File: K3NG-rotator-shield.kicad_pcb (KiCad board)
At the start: 2 copper layers, 81.9 x 70.1 mm, 25 parts, among them J1 Conn_01x08_Socket, J10 Conn_01x01_Pin, J11 Conn_01x10_Socket, J12 Conn_01x01_Pin, J13 Conn_01x01_Pin, J14 Conn_01x01_Pin, J15 Conn_01x01_Pin, J2 Conn_01x04_Socket, J3 Conn_01x02_Pin, J4 Conn_01x04_Socket, J5 Conn_01x01_Pin, J6 Conn_01x07_Socket, J7 Conn_01x06_Socket, J8 Conn_01x08_Socket, J9 Conn_01x06_Socket, U1 DRV8251ADDAR, U2 DRV8251ADDAR

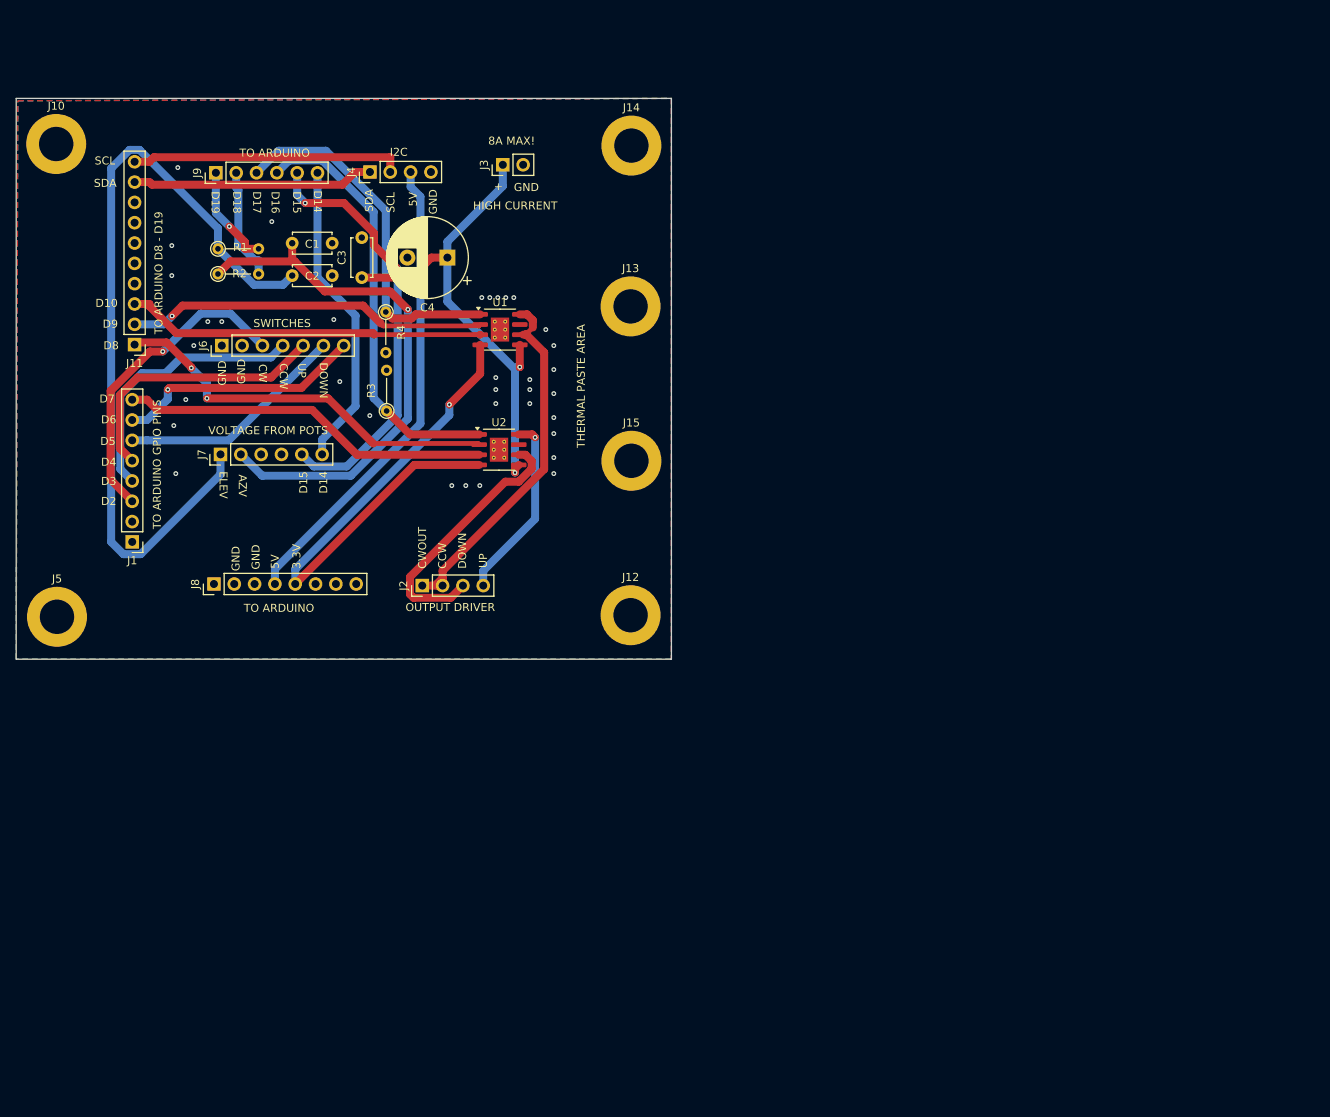
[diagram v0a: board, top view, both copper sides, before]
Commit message: Add files via upload
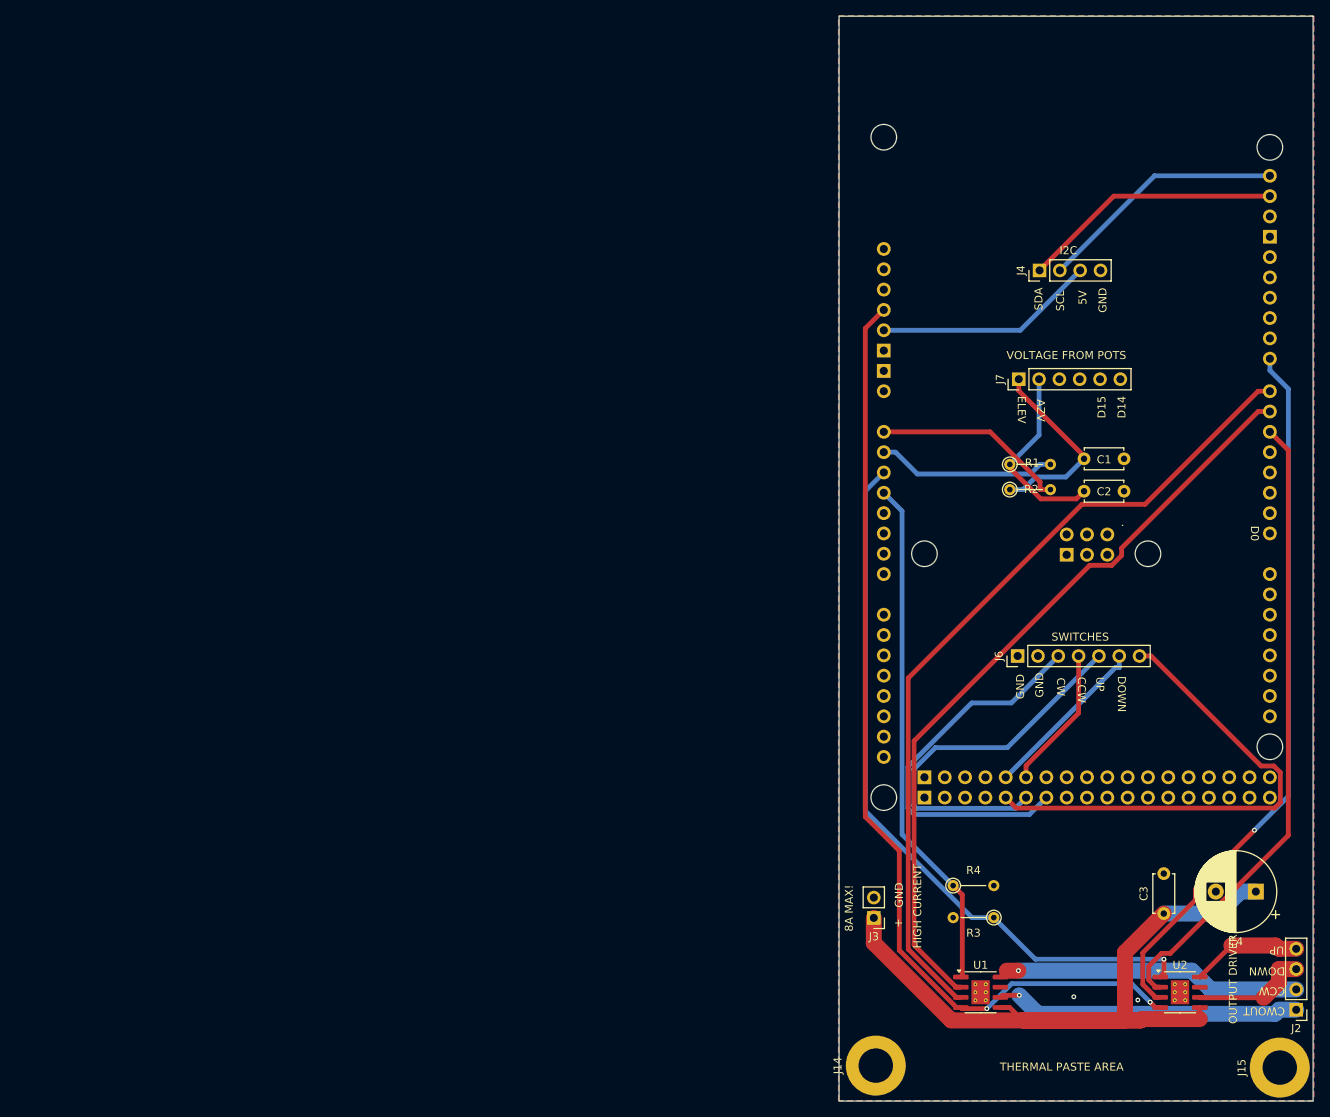
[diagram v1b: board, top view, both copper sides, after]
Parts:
- removed J1, J8: Conn_01x08_Socket, Connector_PinHeader_2.54mm:PinHeader_1x08_P2.54mm_Vertical
- removed J10, J12, J13, J5: Conn_01x01_Pin, MountingHole:MountingHole_4.3mm_M4_DIN965_Pad
- removed J11: Conn_01x10_Socket, Connector_PinHeader_2.54mm:PinHeader_1x10_P2.54mm_Vertical
- removed J9: Conn_01x06_Socket, Connector_PinHeader_2.54mm:PinHeader_1x06_P2.54mm_Vertical
- added A1: Arduino_Mega2560_R3_Shield, sparkfun-electromech:Arduino_Mega2560_R3_K3NG, F.Cu at (131.7, 25.0)
- moved C4 128.4 mm to (180.8, 133.2)
- moved C3 127.9 mm to (169.2, 136.0)
- moved J2 121.4 mm to (185.8, 148.0), turned to 180 degrees
- moved J14 119.0 mm to (133.2, 155.0), turned to 90 degrees
- moved J15 111.0 mm to (183.8, 155.2), turned to 90 degrees
- moved U2 108.8 mm to (171.3, 145.8)
- moved J6 106.8 mm to (151.0, 103.8)
- moved J3 104.9 mm to (133.0, 136.5), turned to 180 degrees
- moved C1 102.6 mm to (159.3, 79.2)
- moved C2 102.6 mm to (159.3, 83.2)
- moved R1 102.6 mm to (150.0, 79.8)
- moved R2 102.6 mm to (150.0, 83.0)
- moved U1 102.3 mm to (146.4, 145.8)
- moved R4 100.8 mm to (142.9, 132.5), turned to 0 degrees
- moved J7 100.2 mm to (151.1, 69.2)
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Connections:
- J2 pad 1: RotateCCW-OUT -> RotateCW-OUT
- J7 pad 1: /ElevationV -> /AzimuthV
- J7 pad 2: /AzimuthV -> /ElevationV
- J7 pad 5: Net-(J7-Pin_5) -> unconnected-(J7-Pin_5-Pad5)
- J7 pad 6: /ACD0 -> unconnected-(J7-Pin_6-Pad6)
- U1 pad 6: RotateCCW-OUT -> RotateCW-OUT
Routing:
- net /ElevationV: track 100.2 -> 23.9 mm
- net RotateCW: track 44.9 -> 103.0 mm
- net Net-(J7-Pin_5): track 53.6 -> 0.00 mm, vias 2 -> 0
- net Vref: track 68.6 -> 120.9 mm, vias 1 -> 2
- net RotateCCW: track 45.3 -> 95.6 mm, vias 1 -> 0
- net VM: track 61.2 -> 108.6 mm, vias 2 -> 0
- net /AzimuthV: track 67.8 -> 24.2 mm, vias 1 -> 0
- net RotateDown: track 46.2 -> 89.6 mm, vias 0 -> 1
- net /ACD0: track 38.9 -> 0.00 mm
- net RotateCW-OUT: track 0.00 -> 38.2 mm, vias 0 -> 1
- net IPRO1: track 53.8 -> 90.7 mm, vias 0 -> 1
- net 5V: track 59.5 -> 27.6 mm
- net Net-(J6-Pin_7): track 31.0 -> 62.5 mm, vias 1 -> 0
- net RotateUP: track 49.6 -> 79.1 mm, vias 2 -> 0
- net IPRO2: track 45.4 -> 64.7 mm
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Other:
- board size 81.9 x 70.1 mm -> 59.2 x 135.6 mm
- board text removed: "3.3V"
- board text removed: "D10"
- board text removed: "D16"
- board text removed: "D17"
- board text removed: "D18"
- board text removed: "D19"
- board text removed: "D2"
- board text removed: "D3"
- board text removed: "D4"
- board text removed: "D5"
- board text removed: "D6"
- board text removed: "D7"
- board text removed: "D8"
- board text removed: "D9"
- board text removed: "TO ARDUINO"
- board text removed: "TO ARDUINO D8 - D19"
- board text removed: "TO ARDUINO GPIO PINS"
